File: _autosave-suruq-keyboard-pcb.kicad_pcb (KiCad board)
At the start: 2 copper layers, 304.8 x 101.2 mm, 150 parts, among them J1 AVR-ISP-6, SW1 Esc, SW10 9, SW11 0, SW12 -, SW13 =, SW14 Back, SW15 Tab, SW16 Q, SW17 W, SW18 E, SW19 R, SW2 1, SW20 T, SW21 Y, SW22 U, SW23 I, SW24 O, SW25 P, SW26 [ {, SW27 ] }, SW28 Enter, SW29 Caps Lock, SW3 2, SW30 A, SW31 S, SW32 D, SW33 F, SW34 G, SW35 H, SW36 J, SW37 K, SW38 L, SW39 ; :, SW4 3, SW40 ' @, SW41 ] }, SW42 Up, SW43 L Shifth, SW44 \ |, SW45 Z, SW46 X, SW47 C, SW48 V, SW49 B, SW5 4, SW50 N, SW51 M, SW52 , <, SW53 . >, SW54 / ?, SW55 R Shift, SW56 Down, SW57 L Ctrl, SW58 Home, SW59 L Alt, SW6 5, SW60 Space, SW61 R Alt, SW62 Fn, SW63 Left, SW64 Right, SW65 SW_Push, SW66 Rotary, SW7 6, SW8 7, SW9 8, U1 PRTR5V0U2X, U2 ATmega32U4-AU, Y1 16MHz

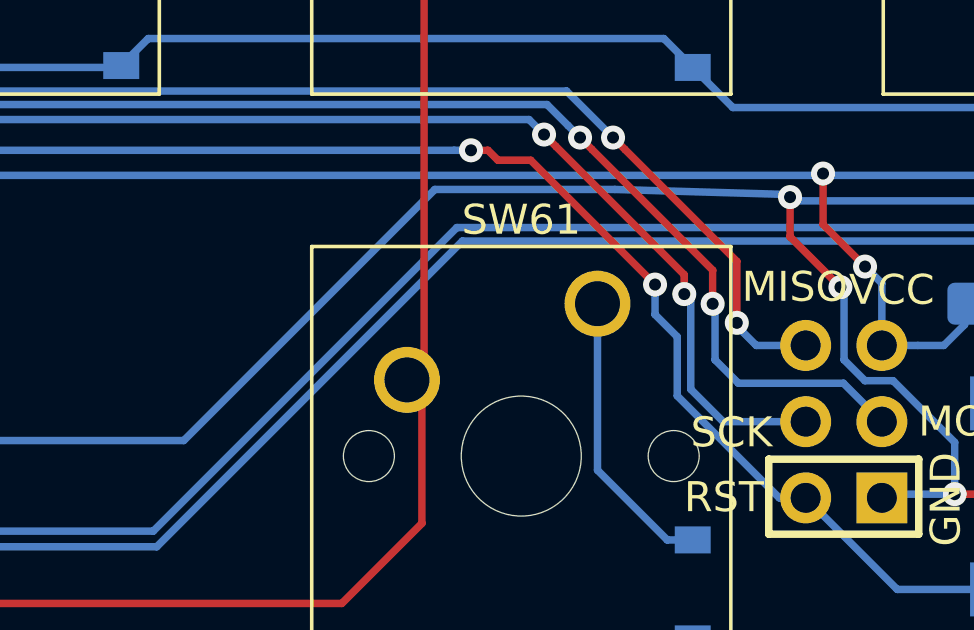
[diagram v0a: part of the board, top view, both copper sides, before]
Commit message: fin routing
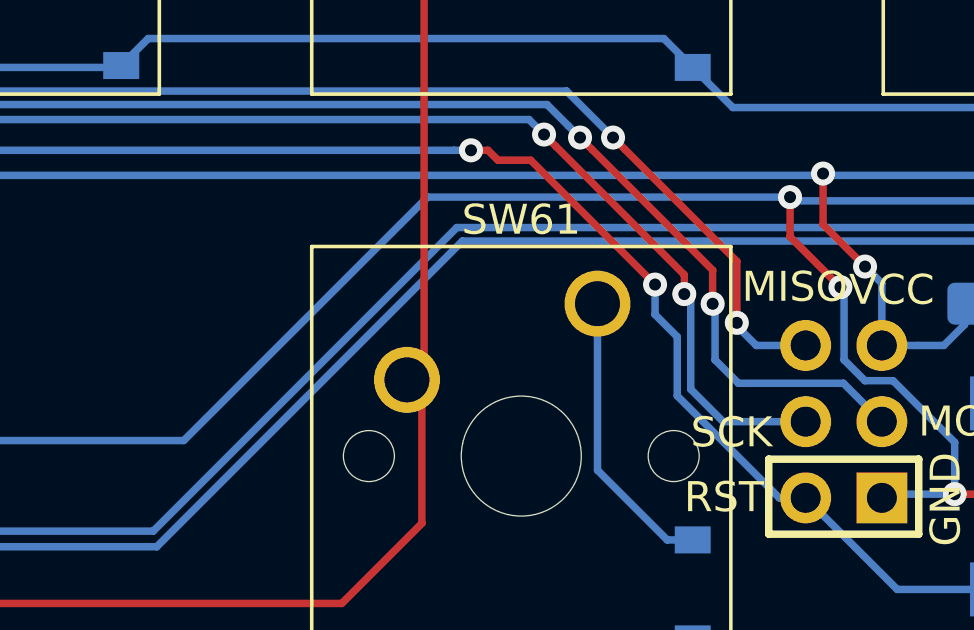
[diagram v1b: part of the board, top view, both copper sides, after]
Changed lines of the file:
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@@
   (via (at 243.75 174.67) (size 0.8) (drill 0.4) (layers F.Cu B.Cu) (net 1))
   (segment (start 243.75 177.6) (end 255.29 177.6) (width 0.25) (layer B.Cu) (net 1))
-  (segment (start 255.29 177.6) (end 263.66 169.23) (width 0.25) (layer B.Cu) (net 1))
-  (segment (start 263.66 169.23) (end 269.66 169.23) (width 0.25) (layer B.Cu) (net 1))
   (via (at 321.11 169.21) (size 0.8) (drill 0.4) (layers F.Cu B.Cu) (net 1))
   (segment (start 350.525 98.425) (end 350.04375 98.425) (width 0.25) (layer B.Cu) (net 1))
@@
   (segment (start 277.218229 172.525) (end 277.1796 172.486371) (width 0.25) (layer B.Cu) (net 1))
   (segment (start 277.3 172.525) (end 277.218229 172.525) (width 0.25) (layer B.Cu) (net 1))
-  (segment (start 269.66 169.23) (end 275.5 169.4) (width 0.25) (layer B.Cu) (net 1))
   (segment (start 277.1796 172.486371) (end 275.5 170.806771) (width 0.25) (layer F.Cu) (net 1))
   (via (at 275.5 169.48501) (size 0.8) (drill 0.4) (layers F.Cu B.Cu) (net 1))
@@
   (segment (start 209.3 99.5) (end 208.1 100.7) (width 0.25) (layer B.Cu) (net 1))
   (segment (start 209.3 99.45) (end 209.3 99.5) (width 0.25) (layer B.Cu) (net 1))
+  (segment (start 263.41499 169.48501) (end 263.3 169.6) (width 0.25) (layer B.Cu) (net 1))
+  (segment (start 275.5 169.48501) (end 263.41499 169.48501) (width 0.25) (layer B.Cu) (net 1))
+  (segment (start 255.29 177.6) (end 263.3 169.6) (width 0.25) (layer B.Cu) (net 1))
   (segment (start 234.85 170.05) (end 235.55 170.05) (width 0.25) (layer B.Cu) (net 2))
   (segment (start 230.38125 173.01875) (end 228.74375 173.01875) (width 0.25) (layer B.Cu) (net 2))
